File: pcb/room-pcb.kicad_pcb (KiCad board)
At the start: 2 copper layers, 50 x 50 mm, 28 parts, among them J2 Conn_01x02, J3 Conn_01x04, J4 Conn_01x05, J5 Conn_01x04, J6 Conn_01x04, U1 COZIR, U2 BH1750FVI-TR, U3 AHT20, U5 ESP32-C6_SUPERMINI_TH

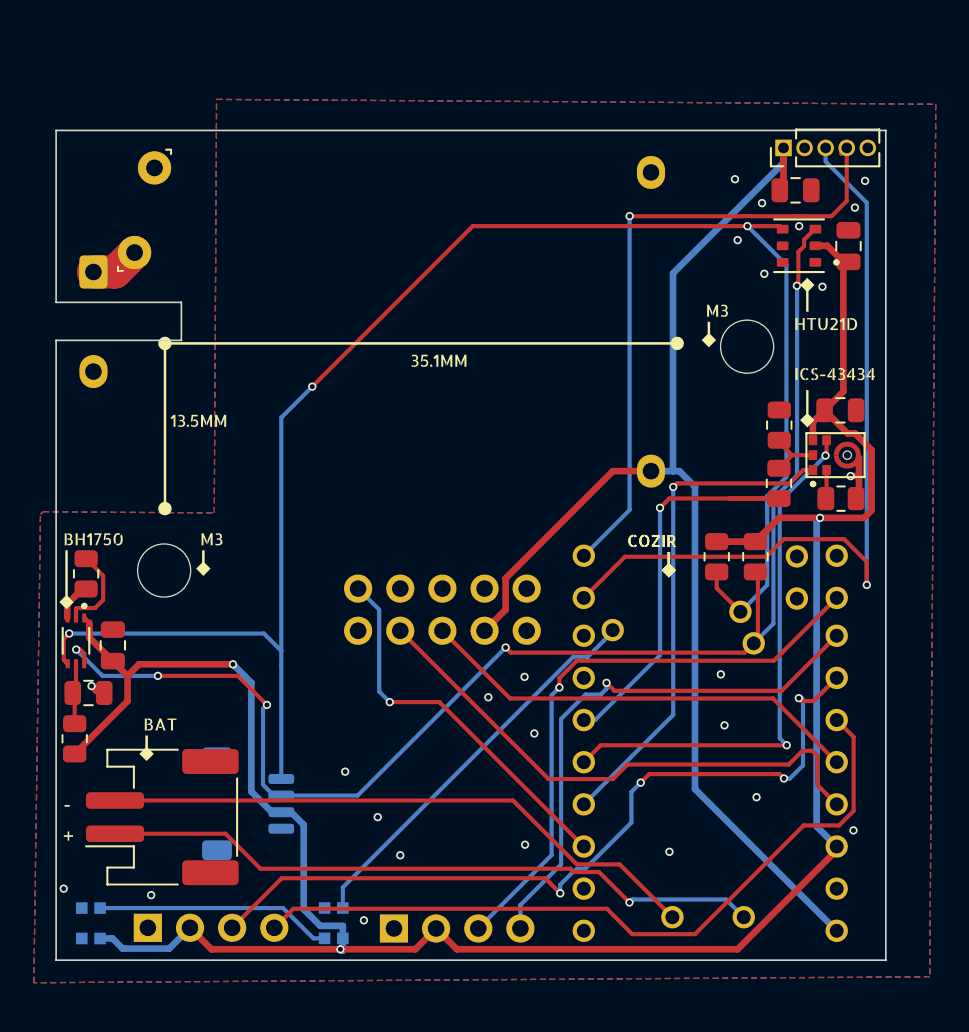
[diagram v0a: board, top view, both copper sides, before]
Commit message: v3
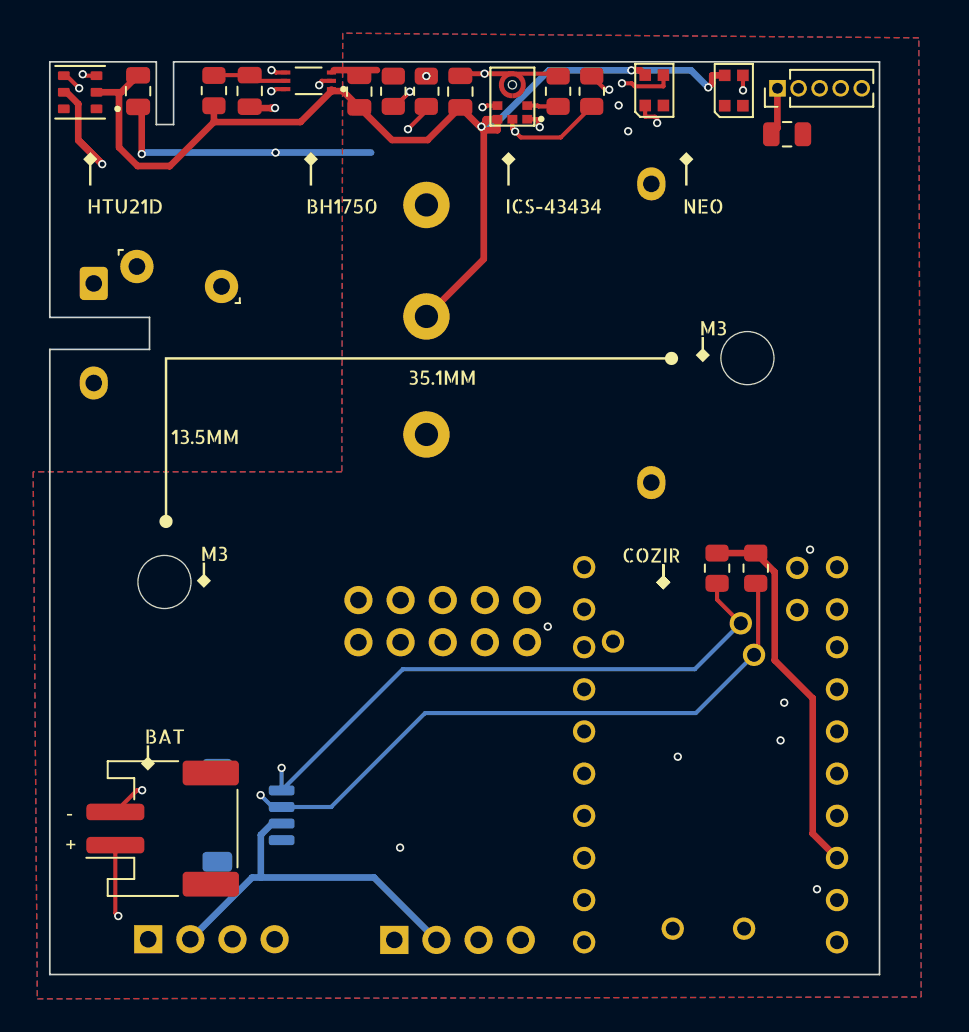
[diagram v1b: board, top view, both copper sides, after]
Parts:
- added TP1: TestPoint, TestPoint:TestPoint_Loop_D2.60mm_Drill1.4mm_Beaded, B.Cu at (121.8, 83.7)
- added TP2: TestPoint, TestPoint:TestPoint_Loop_D2.60mm_Drill1.4mm_Beaded, B.Cu at (121.8, 97.5)
- added TP3: TestPoint, TestPoint:TestPoint_Loop_D2.60mm_Drill1.4mm_Beaded, B.Cu at (121.8, 90.4)
- D1, D2: moved to F.Cu
- moved D2 63.4 mm to (140.3, 76.8)
- moved D1 53.8 mm to (135.5, 76.7)
- moved U3 44.3 mm to (100.9, 76.9)
- moved C5 43.8 mm to (104.4, 76.8), turned to -90 degrees
- moved R1 40.0 mm to (109.0, 76.8)
- moved C1 37.6 mm to (111.2, 76.8), turned to -90 degrees
- moved U2 36.5 mm to (114.7, 76.2), turned to 180 degrees
- moved C6 36.5 mm to (117.8, 76.8)
- moved R5 34.5 mm to (119.8, 76.8), turned to 90 degrees
- moved C2 29.9 mm to (123.8, 76.8), turned to 90 degrees
- moved R2 29.9 mm to (129.7, 76.8), turned to 90 degrees
- moved R3 29.3 mm to (121.8, 76.8)
- moved MK1 29.1 mm to (127.0, 77.1), turned to 180 degrees
- moved R4 26.2 mm to (131.8, 76.8), turned to 90 degrees
- moved F1 8.20 mm to (109.5, 88.6), turned to 180 degrees
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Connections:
- D1 pad 1: +3.3V -> Net-(D1-DOUT)
- D1 pad 2: Net-(D1-DOUT) -> GND
- D1 pad 3: GND -> NEO
- D1 pad 4: NEO -> +3.3V
- D2 pad 1: +3.3V -> unconnected-(D2-DOUT-Pad1)
- D2 pad 2: unconnected-(D2-DOUT-Pad2) -> GND
- D2 pad 3: GND -> Net-(D1-DOUT)
- D2 pad 4: Net-(D1-DOUT) -> +3.3V
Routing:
- net GND: track 6.34 -> 47.2 mm, vias 25 -> 6
- net +3.3V: track 141.2 -> 179.5 mm
- net VCC: track 73.8 -> 102.2 mm
- net CLK: track 32.4 -> 50.2 mm
- net DATA: track 25.5 -> 41.5 mm
- net NEO: track 24.0 -> 38.0 mm, vias 0 -> 1
- net WS: track 30.2 -> 44.0 mm
- net SCL: track 83.9 -> 96.8 mm, vias 5 -> 3
- net Net-(MK1-SD): track 3.59 -> 15.5 mm, vias 0 -> 2
- net BAT-: track 36.5 -> 45.8 mm, vias 0 -> 2
- net EX4: track 45.0 -> 39.1 mm
- net Net-(D1-DOUT): track 14.3 -> 8.59 mm, vias 0 -> 2
- net EX2: track 32.9 -> 38.5 mm
- net SDA: track 100.5 -> 95.4 mm
- net EX3: track 48.0 -> 43.0 mm, vias 4 -> 0
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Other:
- board size 50 x 50 mm -> 50 x 55 mm
- copper layers 2 -> 4
